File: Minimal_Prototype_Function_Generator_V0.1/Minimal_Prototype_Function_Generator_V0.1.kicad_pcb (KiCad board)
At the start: 4 copper layers, 72.3 x 80.6 mm, 170 parts, among them IC1 AD9106BCPZ, IC2 ADP5300ACPZ-1-R7, IC3 ADM7160ACPZN3.3-R7, IC4 LT3472EDD#PBF, IC6 ADM7160ACPZN3.3-R7, IC7 ADM7160ACPZN3.3-R7, IC8 ADM7160ACPZN3.3-R7, IC9 STM32L476VGT6, J1 142-0701-201, J10 SPI_TP_1, J2 142-0701-201, J3 142-0701-201, J4 142-0701-201, J5 142-0701-201, J6 142-0701-201, J7 DEBUG_UART_TP_1, J8 I2C_TP1, J9 USB4500-03-0-A, P5V2_TP1 TestPoint, T1 ADT2-1T+, U1 ADA4817-2ACP, U3 ADA4817-2ACP, Y1 AX3DCF1-156.2500T, Y2 ECS-.327-7-16-C-TR

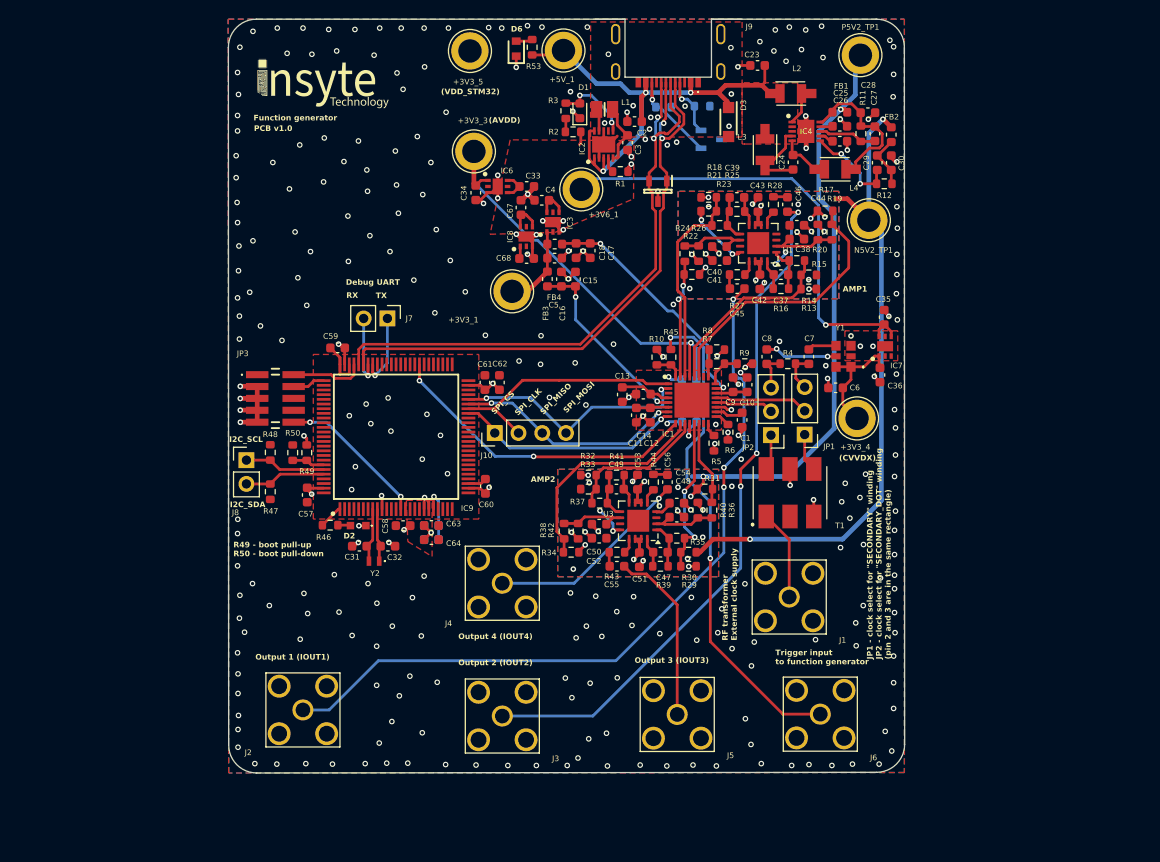
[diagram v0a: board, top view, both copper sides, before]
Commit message: new pcb version
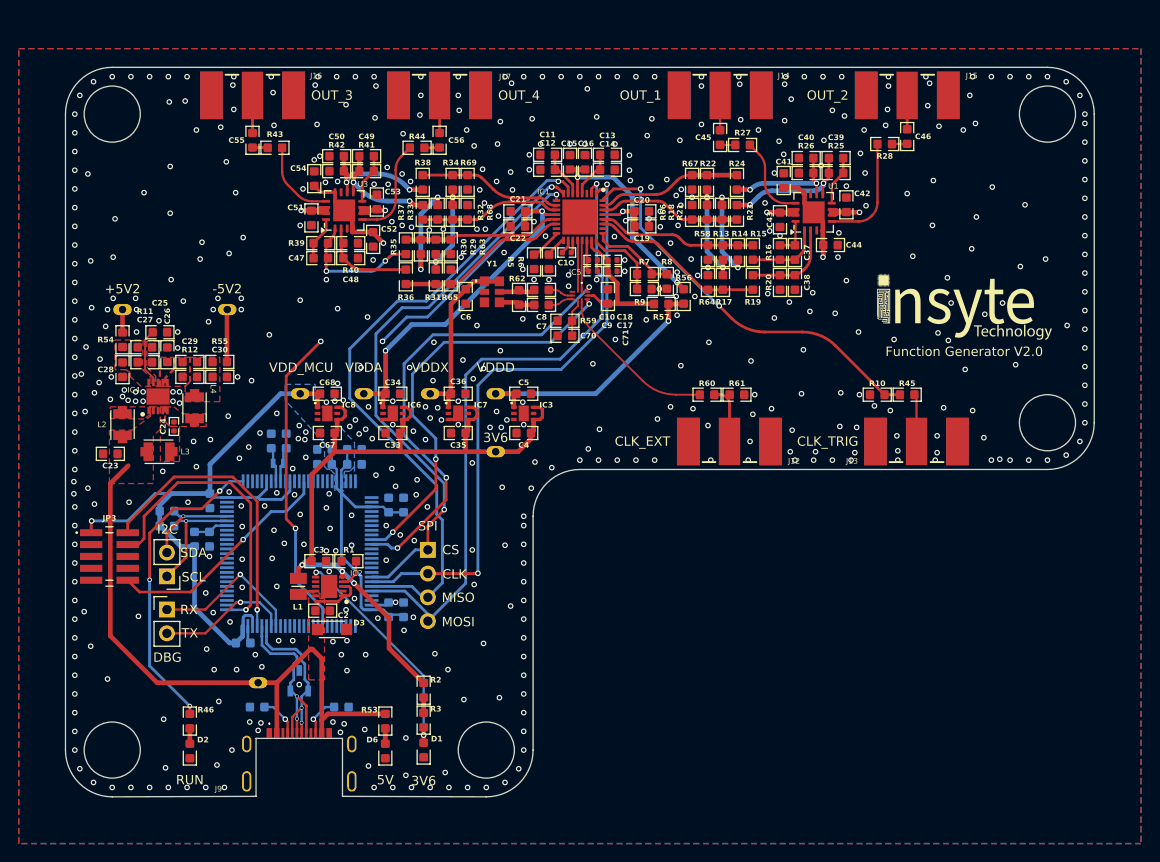
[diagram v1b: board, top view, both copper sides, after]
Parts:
- removed D4: SM05.TCT, Insyte_Footprints:SOT95P237X125-3N
- removed FB1, FB2, FB3, FB4: 1.8K OHM AT 100MEGHZ, Inductor_SMD:L_0603_1608Metric
- removed J1, J2, J3, J4, J5, J6: 142-0701-201, Insyte_Footprints:1420701201
- removed JP1, JP2: Jumper_3_Open, Connector_PinHeader_2.54mm:PinHeader_1x03_P2.54mm_Vertical
- removed R4: 100R, Resistor_SMD:R_0603_1608Metric
- removed T1: ADT2-1T+, Insyte_Footprints:ADT21T
- removed U4: ~, Insyte_Logo_Footprints:15x6_Insyte_Logo
- added C70: 100nF, Insyte_Footprints:C_0603, F.Cu at (86.3, 64.8)
- added C71: 100nF, Insyte_Footprints:C_0603, F.Cu at (90.9, 60.6)
- added G***: LOGO, Insyte_Logo_Footprints:20x8_Insyte_Logo, F.Cu at (128.9, 61.6)
- added IC5: TMUXHS221FRSWR, Insyte_Footprints:TMUXHS221FRSWR, F.Cu at (87.9, 60.5)
- added J12: 142-0701-801, Insyte_Footprints:142-0701-851, F.Cu at (103.9, 76.2)
- added J13: 142-0701-801, Insyte_Footprints:142-0701-851, F.Cu at (123.9, 76.2)
- added J14: 142-0701-801, Insyte_Footprints:142-0701-851, F.Cu at (102.9, 39.1)
- added J15: 142-0701-801, Insyte_Footprints:142-0701-851, F.Cu at (122.9, 39.1)
- added J16: 142-0701-801, Insyte_Footprints:142-0701-851, F.Cu at (52.9, 39.1)
- added J17: 142-0701-801, Insyte_Footprints:142-0701-851, F.Cu at (72.9, 39.1)
- added R54: 0R, Insyte_Footprints:R_0603, F.Cu at (39.0, 65.3)
- added R55: 0R, Insyte_Footprints:R_0603, F.Cu at (49.4, 67.7)
- added R56: 0R, Insyte_Footprints:R_0603, F.Cu at (99.0, 60.6)
- added R57: 0R, Insyte_Footprints:R_0603, F.Cu at (96.6, 61.5)
- added R58: 249R, Insyte_Footprints:R_0603, F.Cu at (101.6, 56.0)
- added R59: 39K, Insyte_Footprints:R_0603, F.Cu at (86.3, 63.2)
- added R60: 100R, Insyte_Footprints:R_0603, F.Cu at (101.5, 71.2)
- added R61: 50R, Insyte_Footprints:R_0603, F.Cu at (104.7, 71.2)
- added R62: 100R, Insyte_Footprints:R_0603, F.Cu at (81.4, 60.8)
- added R63: 249R, Insyte_Footprints:R_0603, F.Cu at (74.1, 55.4)
- added R64: 249R, Insyte_Footprints:R_0603, F.Cu at (101.6, 59.1)
- added R65: 249R, Insyte_Footprints:R_0603, F.Cu at (74.1, 58.5)
- added R66: 249R, Insyte_Footprints:R_0603, F.Cu at (99.9, 51.6)
- added R67: 249R, Insyte_Footprints:R_0603, F.Cu at (99.9, 48.5)
- added R68: 249R, Insyte_Footprints:R_0603, F.Cu at (75.9, 51.6)
- added R69: 249R, Insyte_Footprints:R_0603, F.Cu at (75.9, 48.5)
- +3V3_1, +3V3_3, +3V3_5, +3V6_1, +5V_1, N5V2_TP1, P5V2_TP1: footprint TestPoint:TestPoint_Loop_D3.80mm_Drill2.5mm -> Insyte_Footprints:Testpoint_hole; moved to B.Cu
- +3V3_4: footprint TestPoint:TestPoint_Loop_D3.80mm_Drill2.5mm -> Insyte_Footprints:Testpoint_hole
- C1, C10, C17, C18, C24, C9: footprint Capacitor_SMD:C_0603_1608Metric -> Insyte_Footprints:C_0402
- C11, C12, C13, C14, C15, C16, C2, C23, C25, C26, C27, C28, C29, C3, C30, C33, C34, C35, C36, C37, C38, C39, C4, C40, C41, C44, C45, C46, C47, C48, C49, C5, C50, C52, C54, C55, C56, C67, C68: footprint Capacitor_SMD:C_0603_1608Metric -> Insyte_Footprints:C_0603
- C19, C20, C21, C22: footprint Capacitor_SMD:C_0603_1608Metric -> Insyte_Footprints:C_0603; moved to F.Cu
- C31, C32: footprint Capacitor_SMD:C_0603_1608Metric -> Insyte_Footprints:C_0603; moved to B.Cu
- C42, C43, C51, C53, C6, C7, C8: value 0.1uF -> 100nF; footprint Capacitor_SMD:C_0603_1608Metric -> Insyte_Footprints:C_0603
- C57, C58, C59, C60, C61: value 0.1u -> 0.1uF; footprint Capacitor_SMD:C_0603_1608Metric -> Insyte_Footprints:C_0603; moved to B.Cu
- C62: value 4.7u -> 4.7uF; footprint Capacitor_SMD:C_0603_1608Metric -> Insyte_Footprints:C_0603; moved to B.Cu
- C63: value 0.01u -> 0.01uF; footprint Capacitor_SMD:C_0603_1608Metric -> Insyte_Footprints:C_0603; moved to B.Cu
- C64: value 1u -> 1uF; footprint Capacitor_SMD:C_0603_1608Metric -> Insyte_Footprints:C_0603; moved to B.Cu
- C65: value 0.1u -> 0.1uF; footprint Capacitor_SMD:C_0603_1608Metric -> Insyte_Footprints:C_0603
- C66: value 1u -> 1uF; footprint Capacitor_SMD:C_0603_1608Metric -> Insyte_Footprints:C_0603
- D1: footprint LED_SMD:LED_0603_1608Metric -> Insyte_Footprints:CSL1901MW1
- D5, IC9, J10, Y2: moved to B.Cu
- D6: footprint Insyte_Footprints:LEDC1608X85N -> Insyte_Footprints:CSL1901MW1
- L1: value MLP2016H2R2MT0S1 -> MLP2016V2R2MT0S1
- R1, R10, R11, R12, R13, R14, R15, R16, R17, R18, R19, R20, R21, R22, R23, R24, R25, R26, R27, R28, R29, R3, R30, R31, R32, R33, R34, R35, R36, R37, R38, R39, R40, R41, R42, R43, R44, R45, R46, R5, R51, R52, R53, R6, R7, R8, R9: footprint Resistor_SMD:R_0603_1608Metric -> Insyte_Footprints:R_0603
- R2: value 100R -> 5K; footprint Resistor_SMD:R_0603_1608Metric -> Insyte_Footprints:R_0603
- R47, R48, R49, R50: footprint Resistor_SMD:R_0603_1608Metric -> Insyte_Footprints:R_0603; moved to B.Cu
- moved J9 87.1 mm to (57.9, 111.3), turned to 0 degrees
- moved C28 84.3 mm to (39.0, 68.5), turned to -90 degrees
- moved P5V2_TP1 83.5 mm to (39.0, 62.0)
- moved C27 81.8 mm to (41.4, 67.7), turned to 180 degrees
- moved C23 80.7 mm to (37.7, 77.5)
- moved R51 79.9 mm to (53.4, 104.5), turned to 180 degrees
- moved R11 79.9 mm to (41.4, 66.1), turned to 180 degrees
- moved L2 79.7 mm to (39.0, 74.3), turned to 90 degrees
- moved R12 77.1 mm to (46.2, 69.2)
- moved C29 76.5 mm to (46.2, 67.7), turned to 0 degrees
- moved D6 76.4 mm to (67.1, 109.2)
- moved C25 76.0 mm to (43.0, 64.5)
- moved C26 75.4 mm to (43.8, 66.9), turned to 90 degrees
- moved C30 75.4 mm to (49.4, 69.2), turned to 0 degrees
- moved +5V_1 75.1 mm to (53.5, 102.0), turned to 180 degrees
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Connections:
- IC9 pad 35: unconnected-(IC9-PB0-Pad35) -> /Function Generator/CLOCK_EN
- IC9 pad 36: unconnected-(IC9-PB1-Pad36) -> /Function Generator/CLOCK_SEL
- L4 pad 1: /Power/LT3472EDD/P5V2_VP -> /Power/LT3472EDD/N5V2_VN
- L4 pad 3: /Power/LT3472EDD/P5V2_VP -> /Power/LT3472EDD/N5V2_VN
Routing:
- net GND: track 121.9 -> 8.51 mm, vias 326 -> 542
- net /Power/VDD_STM32: track 14.8 -> 111.0 mm
- net /Output_Stage/Op_Amp_1/AMP_OUT: track 82.3 -> 3.73 mm, vias 3 -> 0
- net /Output_Stage/Op_Amp_1/AMP1_OUT: track 73.8 -> 3.62 mm, vias 3 -> 0
- net /Function Generator/CLOCK_SEL: track 0.00 -> 50.5 mm, vias 0 -> 3
- net Net-(J13-Pad1): track 53.5 -> 5.13 mm, vias 2 -> 0
- net /USB_C/D-: track 66.1 -> 18.4 mm
- net /USB_C/D+: track 66.3 -> 19.6 mm
- net /Function Generator/CLOCK_EN: track 0.00 -> 45.0 mm, vias 0 -> 3
- net /Function Generator/SPI_MISO: track 24.7 -> 69.6 mm, vias 2 -> 1
- net /Function Generator/SPI_MOSI: track 26.2 -> 68.7 mm, vias 2 -> 1
- net /Output_Stage/P5V2: track 89.6 -> 131.4 mm, vias 15 -> 8
- net /Function Generator/Trigger_Input_3V3: track 2.98 -> 43.7 mm, vias 0 -> 2
- net /Function Generator/SPI_CLK: track 26.5 -> 65.0 mm, vias 0 -> 2
- net /Output_Stage/N5V2: track 84.0 -> 122.2 mm, vias 8 -> 6
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- added copper zone on F.Cu, net /Power/LT3472EDD/N5V2_VN
- added copper zone on F.Cu, net /Power/LT3472EDD/P5V2_VP
- added copper zone on B.Cu, net /Power/VDD_STM32
- added copper zone on F.Cu, net Net-(IC4-DN)
- added copper zone on F.Cu, net Net-(IC4-FBN)
- added copper zone on F.Cu, net Net-(IC4-FBP)
- added copper zone on F.Cu, net Net-(IC4-SSN)
- added copper zone on F.Cu, net Net-(IC4-SWN)
- added copper zone on F.Cu, net Net-(IC4-SWP)
- removed copper zone on F.Cu, net /Output_Stage/N5V2
- removed copper zone on B.Cu, net /Output_Stage/P5V2
- removed copper zone on F.Cu, net /Power/ADM7160ACPZN3.3_1/+3V6
- removed copper zone on F.Cu, net /Power/VDD_STM32
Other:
- board size 72.3 x 80.6 mm -> 110 x 78 mm
- board text added: "+5V2"
- board text added: "-5V2"
- board text added: "3V6"
- board text added: "5V"
- board text added: "CLK"
- board text added: "CLK_EXT"
- board text added: "CLK_TRIG"
- board text added: "CS"
- board text added: "DBG"
- board text added: "Function Generator V2.0"
- board text added: "I2C"
- board text added: "MISO"
- board text added: "MOSI"
- board text added: "OUT_1"
- board text added: "OUT_2"
- board text added: "OUT_3"
- board text added: "OUT_4"
- board text added: "RUN"
- board text added: "SCL"
- board text added: "SDA"
- board text added: "SPI"
- board text added: "VDDA"
- board text added: "VDDD"
- board text added: "VDDX"
- board text added: "VDD_MCU"
- board text removed: "(AVDD)"
- board text removed: "(CVVDX)"
- board text removed: "(VDD_STM32)"
- board text removed: "AMP1"
- board text removed: "AMP2"
- board text removed: "Debug UART"
- board text removed: "Function generator"
- board text removed: "I2C_SCL"
- board text removed: "I2C_SDA"
- board text removed: "JP1 - clock select for {dblquote}SECONDARY{dblquote} winding JP2 - clock select for {dblquote}SECONDARY_DOT{dblquote} winding (pin 2 and 3 are in the same rectangle)"
- board text removed: "Output 1 (IOUT1)"
- board text removed: "Output 2 (IOUT2)"
- board text removed: "Output 3 (IOUT3)"
- board text removed: "Output 4 (IOUT4)"
- board text removed: "PCB v1.0"
- board text removed: "R49 - boot pull-up"
- board text removed: "R50 - boot pull-down"
- board text removed: "RF transformer External clock supply"
- board text removed: "SPI_CLK"
- board text removed: "SPI_CS"
- board text removed: "SPI_MISO"
- board text removed: "SPI_MOSI"
- board text removed: "Trigger input to function generator"
